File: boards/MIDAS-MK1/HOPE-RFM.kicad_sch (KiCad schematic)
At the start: 1 part, among them U1 RFM96W-433S2

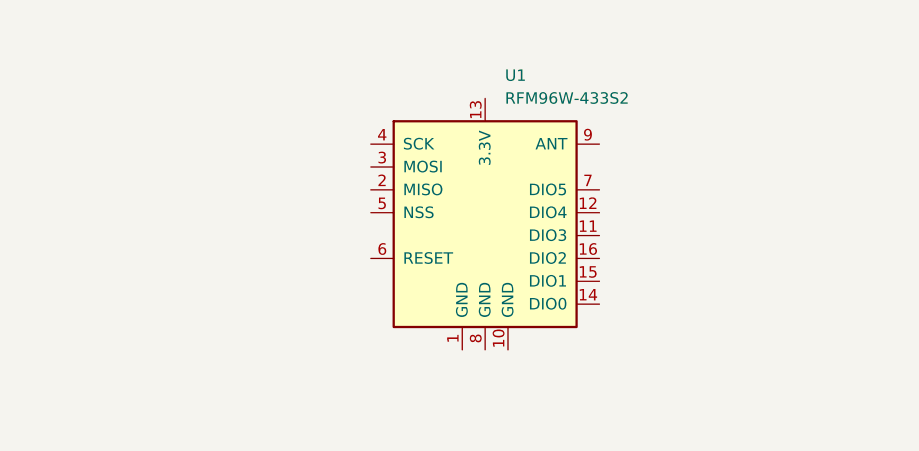
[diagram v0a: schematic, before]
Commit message: Finished HOPE sch
Finished HOPE sch
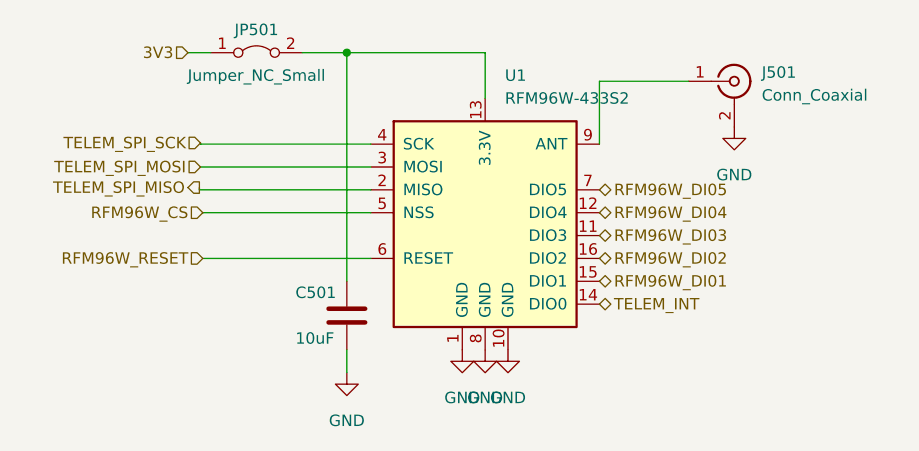
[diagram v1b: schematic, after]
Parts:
- added C501: 10uF, Capacitor_SMD:C_0805_2012Metric, symbol D24V50F5:C
- added J501: Conn_Coaxial, symbol Connector:Conn_Coaxial
- added JP501: Jumper_NC_Small, Jumper:SolderJumper-2_P1.3mm_Bridged_RoundedPad1.0x1.5mm, symbol Jumper:Jumper_2_Bridged
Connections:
- net GND: now reaches U1.1 (GND)
- net GND: now also U1.10 (GND), U1.8 (GND), C501.2, J501.2 (Ext)
- net RFM96W_DI03: now reaches U1.11 (DIO3)
- net RFM96W_DI04: now reaches U1.12 (DIO4)
- net at U1.13 (3.3V): now also C501.1, JP501.2 (B)
- net TELEM_INT: now reaches U1.14 (DIO0)
- net RFM96W_DI01: now reaches U1.15 (DIO1)
- net RFM96W_DI02: now reaches U1.16 (DIO2)
- net TELEM_SPI_MISO: now reaches U1.2 (MISO)
- net TELEM_SPI_MOSI: now reaches U1.3 (MOSI)
- net TELEM_SPI_SCK: now reaches U1.4 (SCK)
- net RFM96W_CS: now reaches U1.5 (NSS)
- net RFM96W_RESET: now reaches U1.6 (RESET)
- net RFM96W_DI05: now reaches U1.7 (DIO5)
- net at U1.9 (ANT): now also J501.1 (In)
- new net 3V3: JP501.1 (A)
